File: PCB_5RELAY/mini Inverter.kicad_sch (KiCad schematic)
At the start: 41 parts, among them IC1 ULN2003, J1 Conn_01x05_Pin, J2 Conn_01x03_Pin, U1 HLK-PM12, U2 L7805, U3 AMS1117, U4 ESP32-WROOM-32

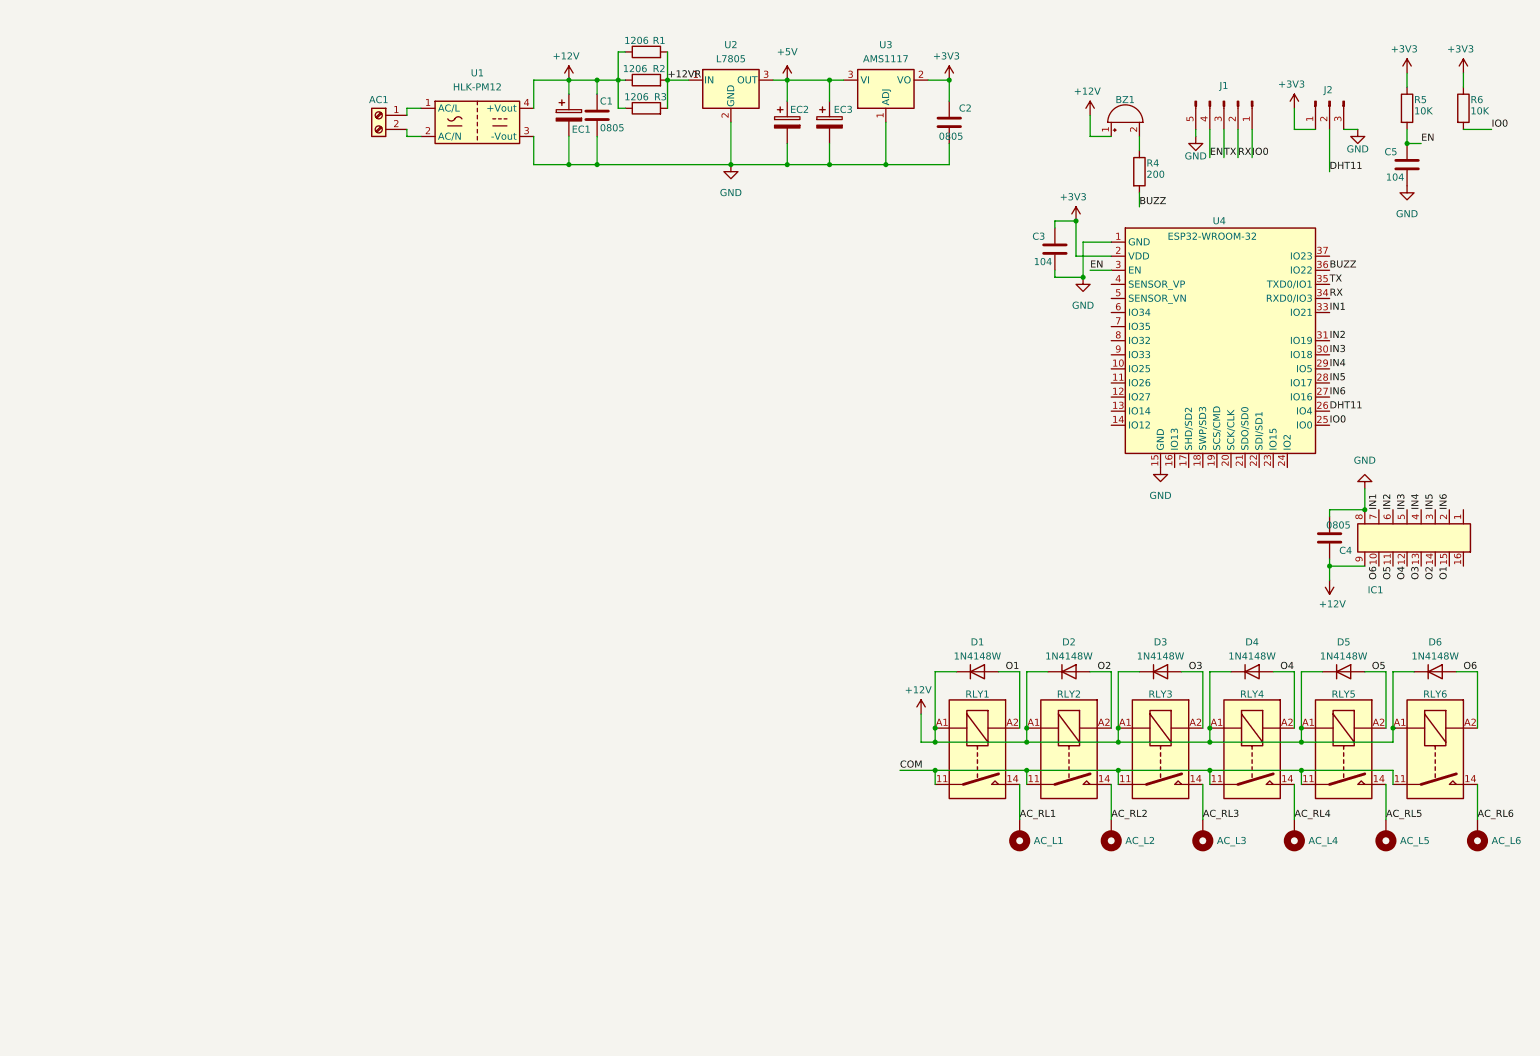
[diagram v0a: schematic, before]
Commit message: 091026
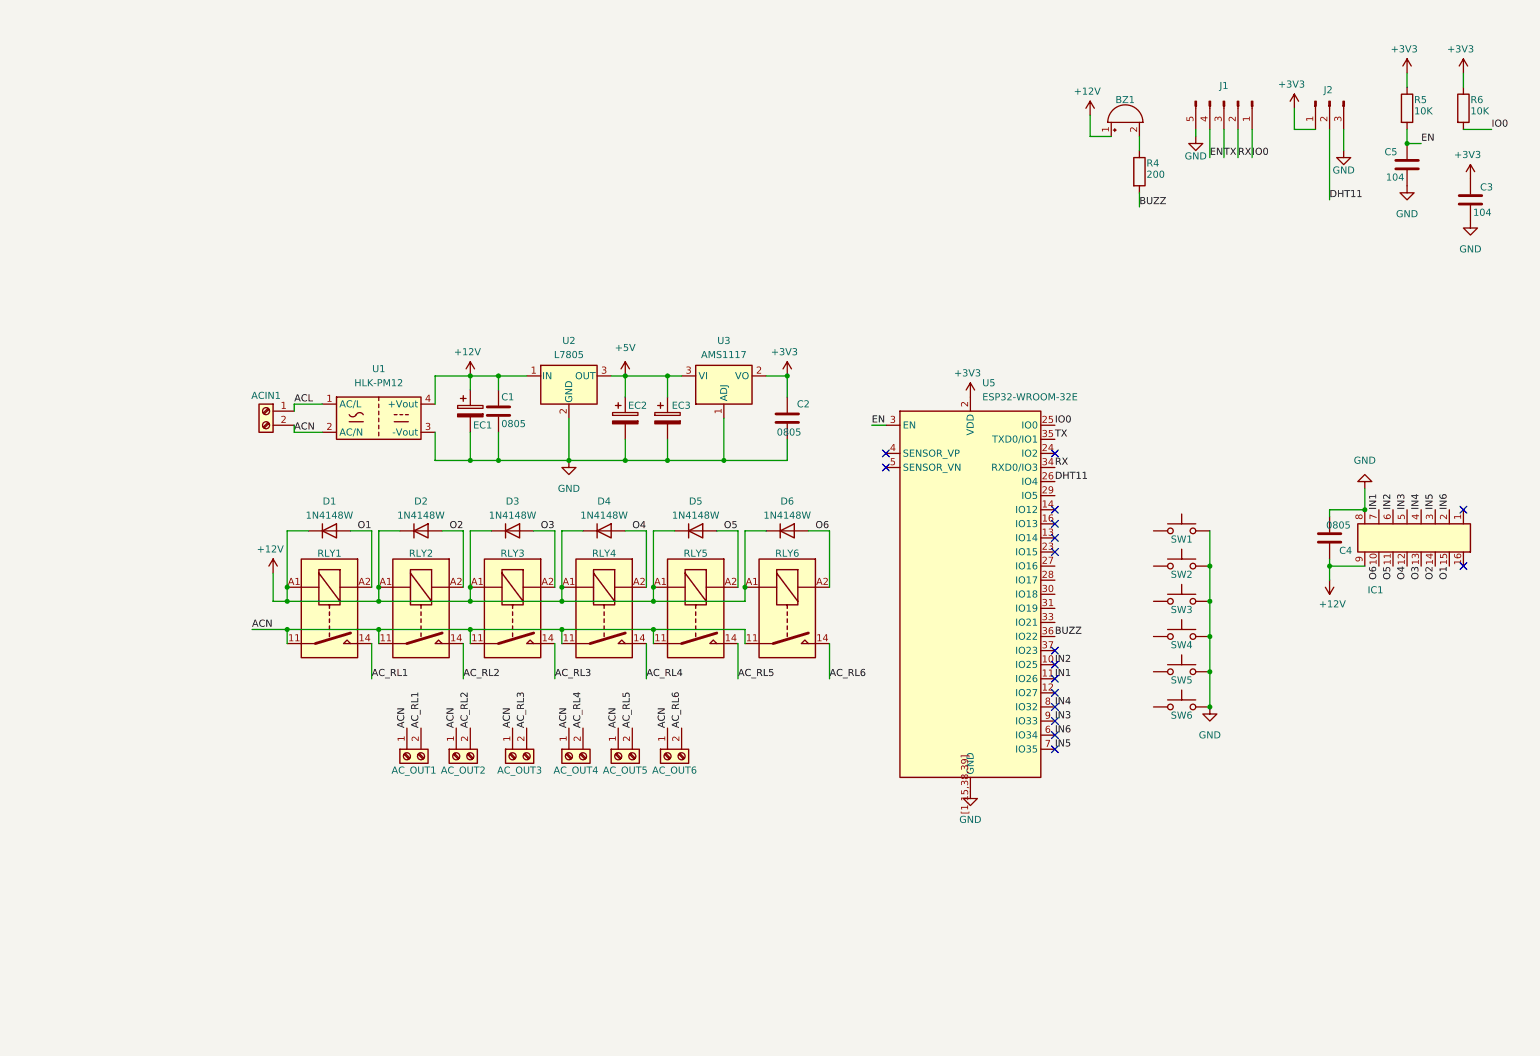
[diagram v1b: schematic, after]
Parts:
- removed AC_L1, AC_L2, AC_L3, AC_L4, AC_L5, AC_L6: MountingHole_Pad, 1_Mycustomfootprint:PAD_AC, symbol Mechanical:MountingHole_Pad
- removed R1, R2, R3: 1206, Resistor_SMD:R_1206_3216Metric, symbol Device:R
- removed U4: ESP32-WROOM-32, RF_Module:ESP32-WROOM-32, symbol RF_Module:ESP32-WROOM-32
- added AC_OUT1, AC_OUT2, AC_OUT3, AC_OUT4, AC_OUT5, AC_OUT6: Screw_Terminal_01x02, 1_Mycustomfootprint:TerminalBlock_Phoenix_MKDS-1,5-2_1x02_P5.00mm_Horizontal, symbol Connector:Screw_Terminal_01x02
- added SW1, SW2, SW3, SW4, SW5, SW6: Nút Nhấn 6x6mm Cao 5.5mm 2 Chân, symbol Switch:SW_Push
- added U5: ESP32-WROOM-32E, 1_Mycustomfootprint:ESP32-WROOM-32E, symbol 1_Mycustomsymbol:ESP32-WROOM-32E
- EC2, EC3: footprint Capacitor_THT:CP_Radial_D6.3mm_P2.50mm -> 1_Mycustomfootprint:CP_Radial_D5.0mm_P2.50mm
- J1: footprint Connector_PinHeader_2.54mm:PinHeader_1x05_P2.54mm_Vertical -> 1_Mycustomfootprint:PinHeader_1x05_P2.54mm_Vertical
- J2: footprint Connector_PinHeader_2.54mm:PinHeader_1x03_P2.54mm_Vertical -> 1_Mycustomfootprint:DHT11
- renumbered AC1 to ACIN1
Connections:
- net +12VR is gone; now on net +12V: U2.1 (IN)
- net COM is gone; now on net ACN: RLY1.11, RLY2.11, RLY3.11, RLY4.11, RLY5.11, RLY6.11
- net +3V3: now also U5.2 (VDD)
- net AC_RL1: now also AC_OUT1.2 (Pin_2)
- net AC_RL2: now also AC_OUT2.2 (Pin_2)
- net AC_RL3: now also AC_OUT3.2 (Pin_2)
- net AC_RL4: now also AC_OUT4.2 (Pin_2)
- net AC_RL5: now also AC_OUT5.2 (Pin_2)
- net AC_RL6: now also AC_OUT6.2 (Pin_2)
- net BUZZ: now also U5.36 (IO22)
- net DHT11: now also U5.26 (IO4)
- net EN: now also U5.3 (EN)
- net GND: now also SW1.2, SW2.2, SW3.2, SW4.2, SW5.2, SW6.2, U5.[1,15,38,39] (GND)
- net IN1: now also U5.11 (IO26)
- net IN2: now also U5.10 (IO25)
- net IN3: now also U5.9 (IO33)
- net IN4: now also U5.8 (IO32)
- net IN5: now also U5.7 (IO35)
- net IN6: now also U5.6 (IO34)
- net IO0: now also U5.25 (IO0)
- net RX: now also U5.34 (RXD0/IO3)
- net TX: now also U5.35 (TXD0/IO1)
- net ACL: now reaches ACIN1.1 (Pin_1), U1.1 (AC/L)
- net ACN: now reaches ACIN1.2 (Pin_2), U1.2 (AC/N)
- net ACN: now also AC_OUT1.1 (Pin_1), AC_OUT2.1 (Pin_1), AC_OUT3.1 (Pin_1), AC_OUT4.1 (Pin_1), AC_OUT5.1 (Pin_1), AC_OUT6.1 (Pin_1)
- no-connect marks 0 -> 17
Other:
- moved on the sheet: ACIN1, C1, C2, C3, D1, D2, D3, D4, D5, D6, EC1, EC2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

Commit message: 151026
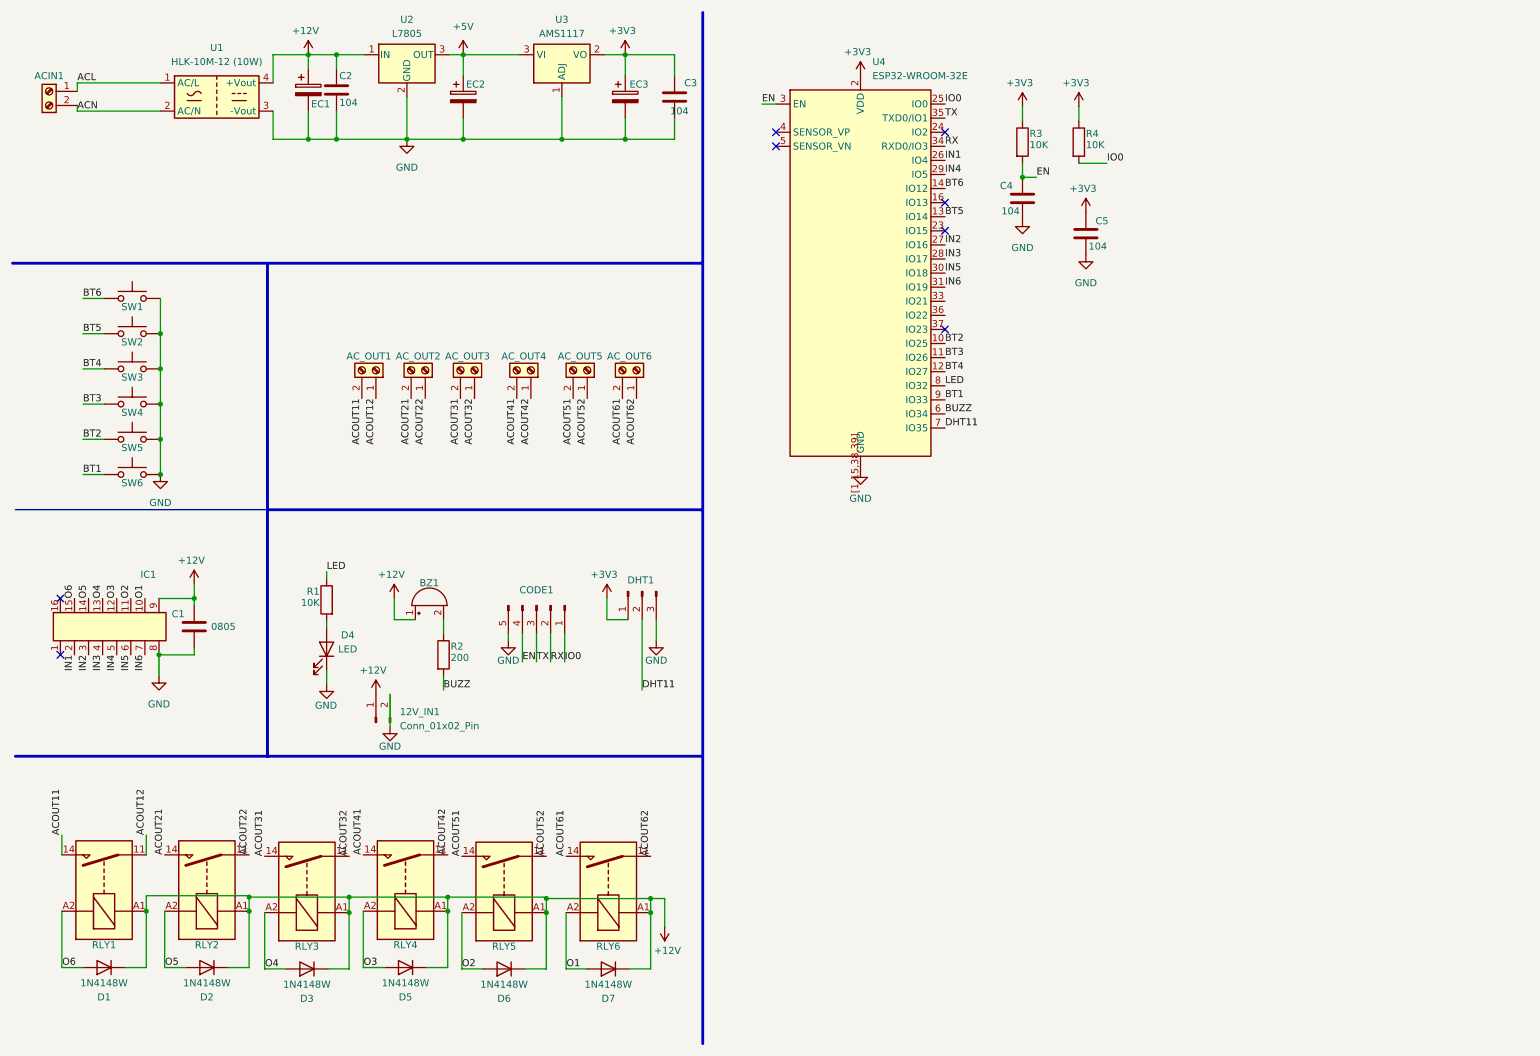
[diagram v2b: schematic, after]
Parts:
- added 12V_IN1: Conn_01x02_Pin, TerminalBlock:TerminalBlock_Xinya_XY308-2.54-2P_1x02_P2.54mm_Horizontal, symbol Connector:Conn_01x02_Pin
- added D4: LED, 1_Mycustomfootprint:LED_0805_2012Metric, symbol Device:LED
- added R1: 10K, Resistor_SMD:R_0805_2012Metric, symbol Device:R
- C2: renamed from C1; value 0805 -> 104
- C3: renamed from C2; value 0805 -> 104
- D1: renamed from D6; footprint Diode_SMD:D_SOD-123 -> 1_Mycustomfootprint:D_SOD-123
- D2: renamed from D5; footprint Diode_SMD:D_SOD-123 -> 1_Mycustomfootprint:D_SOD-123
- D3: renamed from D4; footprint Diode_SMD:D_SOD-123 -> 1_Mycustomfootprint:D_SOD-123
- D5: renamed from D3; footprint Diode_SMD:D_SOD-123 -> 1_Mycustomfootprint:D_SOD-123
- D6: renamed from D2; footprint Diode_SMD:D_SOD-123 -> 1_Mycustomfootprint:D_SOD-123
- D7: renamed from D1; footprint Diode_SMD:D_SOD-123 -> 1_Mycustomfootprint:D_SOD-123
- EC1: value C_Polarized -> 220µF/25V; footprint Capacitor_THT:CP_Radial_D10.0mm_P5.00mm -> 1_Mycustomfootprint:CP_Radial_D5.0mm_P2.50mm
- EC2: value C_Polarized -> 47µF
- EC3: value C_Polarized -> 10µF
- SW1, SW2, SW3, SW4, SW5, SW6: footprint (none) -> 1_Mycustomfootprint:Nút Nhấn 6x6mm Cao 5.5mm
- U1: value HLK-PM12 -> HLK-10M-12 (10W)
- U2: footprint Package_TO_SOT_SMD:TO-252-2 -> 1_Mycustomfootprint:TO-252-2
- U3: footprint Package_TO_SOT_SMD:SOT-223-3_TabPin2 -> 1_Mycustomfootprint:SOT-223-3_TabPin2
- renumbered AC_OUT6 to AC_OUT1, AC_OUT5 to AC_OUT2, AC_OUT4 to AC_OUT3, AC_OUT3 to AC_OUT4, AC_OUT2 to AC_OUT5, AC_OUT1 to AC_OUT6, C4 to C1, C5 to C4, C3 to C5, J1 to CODE1, J2 to DHT1, R4 to R2, R5 to R3, R6 to R4, RLY6 to RLY1, RLY5 to RLY2, RLY4 to RLY3, RLY3 to RLY4, RLY2 to RLY5, RLY1 to RLY6, U5 to U4
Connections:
- net +12V: now also 12V_IN1.1 (Pin_1)
- net +3V3: now also EC3.1
- net +5V: no longer EC3.1
- net ACN: no longer AC_OUT1.1 (Pin_1), AC_OUT2.1 (Pin_1), AC_OUT3.1 (Pin_1), AC_OUT4.1 (Pin_1), AC_OUT5.1 (Pin_1), AC_OUT6.1 (Pin_1), RLY1.11, RLY2.11, RLY3.11, RLY4.11, RLY5.11, RLY6.11
- net BUZZ: now also U4.6 (IO34); no longer U4.36 (IO22)
- net DHT11: now also U4.7 (IO35); no longer U4.26 (IO4)
- net GND: now also 12V_IN1.2 (Pin_2), D4.1 (K)
- net IN1: now also IC1.2, U4.26 (IO4); no longer IC1.7, U4.11 (IO26)
- net IN2: now also IC1.3, U4.27 (IO16); no longer IC1.6, U4.10 (IO25)
- net IN3: now also IC1.4, U4.28 (IO17); no longer IC1.5, U4.9 (IO33)
- net IN4: now also IC1.5, U4.29 (IO5); no longer IC1.4, U4.8 (IO32)
- net IN5: now also IC1.6, U4.30 (IO18); no longer IC1.3, U4.7 (IO35)
- net IN6: now also IC1.7, U4.31 (IO19); no longer IC1.2, U4.6 (IO34)
- net O1: now also IC1.10; no longer IC1.15
- net O2: now also IC1.11; no longer IC1.14
- net O3: now also IC1.12; no longer IC1.13
- net O4: now also IC1.13; no longer IC1.12
- net O5: now also IC1.14; no longer IC1.11
- net O6: now also IC1.15; no longer IC1.10
- net BT6: now reaches SW1.1
- net BT6: now also U4.14 (IO12)
- net BT2: now reaches SW5.1
- net BT2: now also U4.10 (IO25)
- net BT4: now reaches SW3.1
- net BT4: now also U4.12 (IO27)
- net BT5: now reaches U4.13 (IO14)
- net BT5: now also SW2.1
- net BT1: now reaches SW6.1
- net BT1: now also U4.9 (IO33)
- net BT3: now reaches SW4.1
- net BT3: now also U4.11 (IO26)
- net AC_RL1 renamed ACOUT61
- net AC_RL2 renamed ACOUT51
- net AC_RL3 renamed ACOUT41
- net AC_RL4 renamed ACOUT31
- net AC_RL5 renamed ACOUT21
- net AC_RL6 renamed ACOUT11
- new net: D4.2 (A), R1.2
- new net ACOUT12: AC_OUT1.1 (Pin_1), RLY1.11
- new net ACOUT22: AC_OUT2.1 (Pin_1), RLY2.11
- new net ACOUT32: AC_OUT3.1 (Pin_1), RLY3.11
- new net ACOUT42: AC_OUT4.1 (Pin_1), RLY4.11
- new net ACOUT52: AC_OUT5.1 (Pin_1), RLY5.11
- new net ACOUT62: AC_OUT6.1 (Pin_1), RLY6.11
- new net LED: R1.1, U4.8 (IO32)
- no-connect marks 17 -> 8
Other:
- moved on the sheet: ACIN1, AC_OUT1, AC_OUT2, AC_OUT3, AC_OUT4, AC_OUT5, AC_OUT6, BZ1, C1, C2, C3, C4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
